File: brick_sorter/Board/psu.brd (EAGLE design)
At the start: 51.5 x 60.4 mm, 14 parts, among them IC1 LM2574N-3.3, IC2-12V 786TV, IC2-6V 786TV

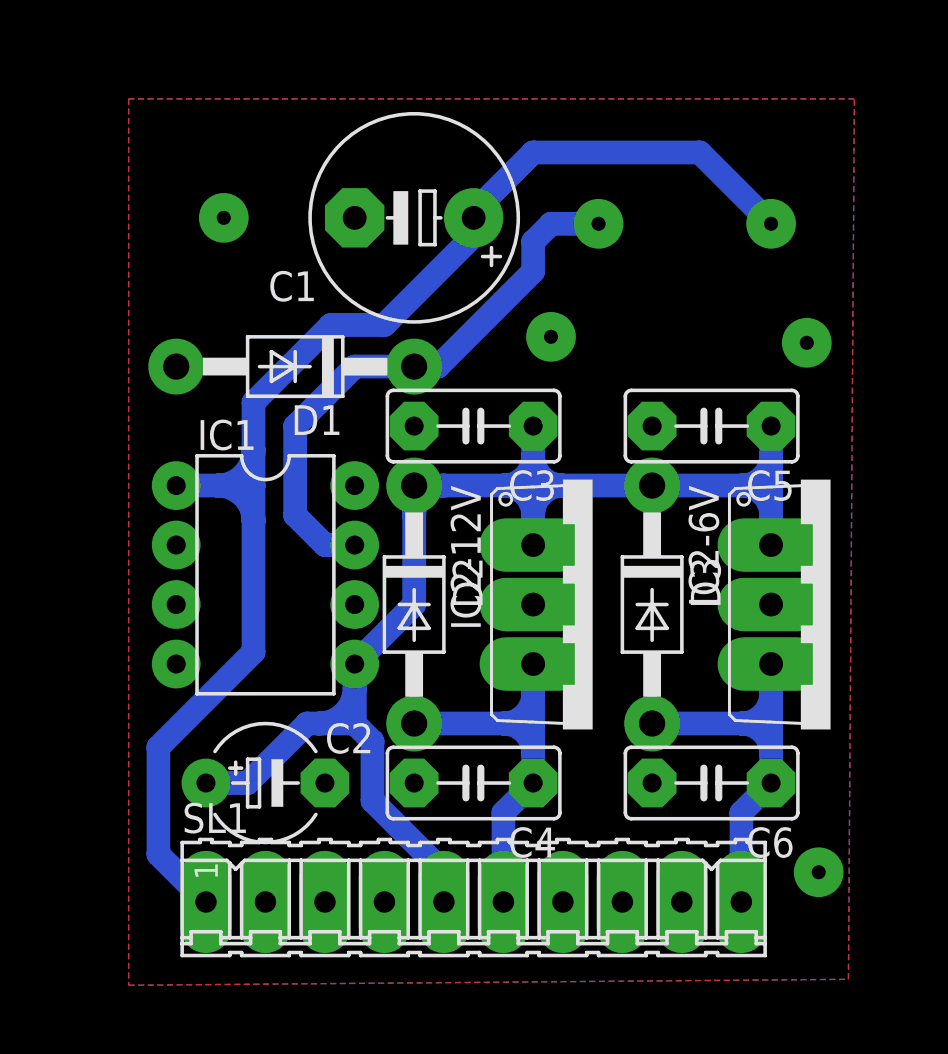
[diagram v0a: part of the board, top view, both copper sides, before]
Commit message: Board v2.1 - now reversed
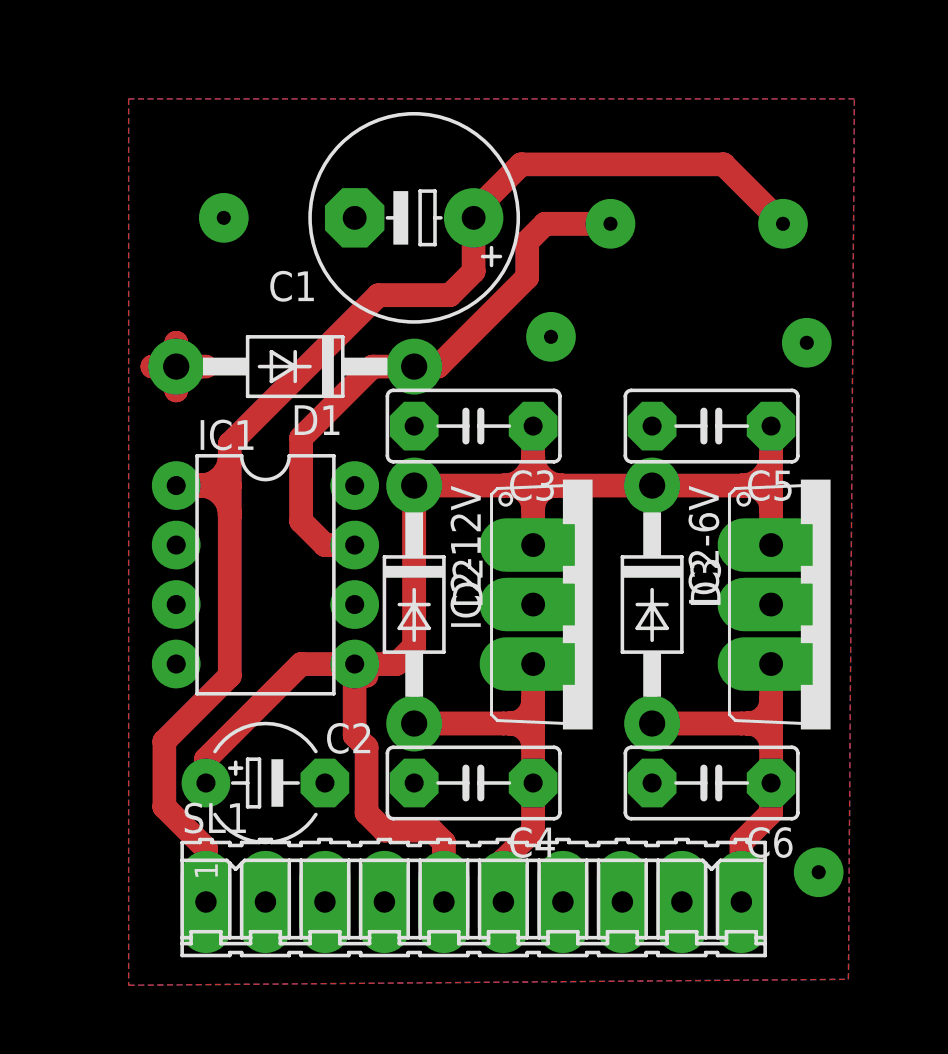
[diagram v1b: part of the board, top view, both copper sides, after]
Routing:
- net N$1: track 0.00 -> 5.90 mm
- net 5V: track 59.8 -> 58.4 mm, vias 1 -> 0
- net 6V: track 19.4 -> 18.6 mm
- net 15V: track 67.9 -> 68.6 mm
- net 12V: track 19.4 -> 18.7 mm
- net LM_OUT: vias 1 -> 0
